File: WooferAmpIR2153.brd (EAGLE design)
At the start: 142.2 x 47.3 mm, 71 parts

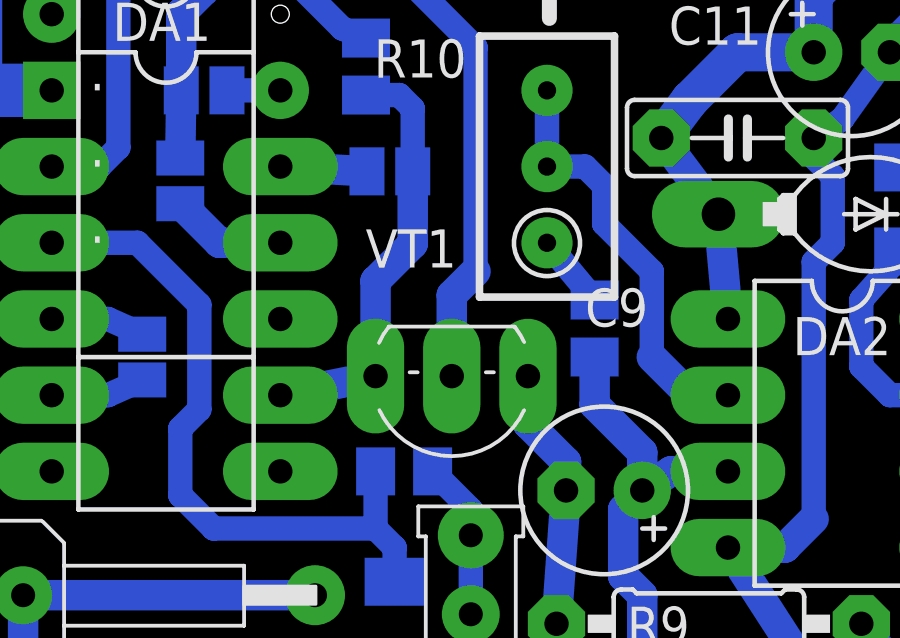
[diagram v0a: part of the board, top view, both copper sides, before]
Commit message: rel4
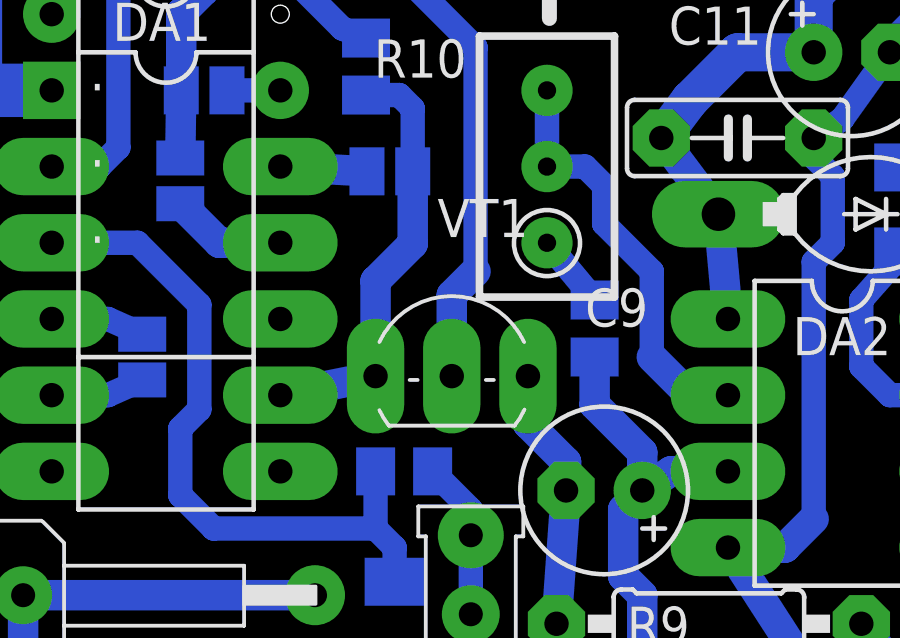
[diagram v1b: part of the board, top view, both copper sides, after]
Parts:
- VT1: device transistor:TO92-CBE -> m_transistor:TO92
- moved VT1 1.27 mm to (26.4, 17.1), turned to 0 degrees
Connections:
- net CO: now also VT1.1; no longer VT1.E
- net GND: now also VT1.2; no longer VT1.B
- net N$50: now also VT1.3; no longer VT1.C
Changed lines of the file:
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@@
 </autorouter>
 <elements>
-<element name="VT1" library="transistor" package="TO92-CBE" value="2N5401" x="26.3525" y="15.875" smashed="yes" rot="R180">
-<attribute name="NAME" x="26.51125" y="20.7645" size="1.27" layer="25" ratio="10" rot="R180"/>
-<attribute name="VALUE" x="23.1775" y="17.9705" size="1.27" layer="27" ratio="10"/>
+<element name="VT1" library="m_transistor" package="TO92" value="2N5401" x="26.3525" y="17.145" smashed="yes">
+<attribute name="NAME" x="25.87625" y="20.5105" size="1.27" layer="25" ratio="10"/>
+<attribute name="VALUE" x="29.5275" y="15.0495" size="1.27" layer="27" ratio="10" rot="R180"/>
 </element>
 <element name="C10" library="resistor" package="C075-032X103" value="750" x="35.2425" y="4.7625" smashed="yes">
@@
 <element name="R11" library="resistor" package="M0805" value="750" x="31.115" y="17.4625" smashed="yes" rot="MR270">
 <attribute name="NAME" x="26.63825" y="18.95475" size="1.27" layer="26" ratio="10" rot="MR180"/>
-<attribute name="VALUE" x="26.0731" y="17.78" size="1.27" layer="28" ratio="10" rot="MR0"/>
+<attribute name="VALUE" x="26.0731" y="18.0975" size="1.27" layer="28" ratio="10" rot="MR0"/>
 </element>
 <element name="C11" library="resistor" package="C050-025X075" value="100n" x="35.8775" y="23.8125" smashed="yes">
@@
 <contactref element="C17" pad="2"/>
 <contactref element="VT2" pad="2"/>
-<contactref element="VT1" pad="B"/>
+<contactref element="VT1" pad="2"/>
 <contactref element="R12" pad="1"/>
 <contactref element="C3" pad="1"/>
@@
 </signal>
 <signal name="N$50">
-<contactref element="VT1" pad="C"/>
+<contactref element="VT1" pad="3"/>
 <contactref element="R9" pad="1"/>
 <contactref element="C9" pad="-"/>
@@
 <contactref element="R8" pad="1"/>
 <contactref element="SJ3" pad="2"/>
-<contactref element="VT1" pad="E"/>
+<contactref element="VT1" pad="1"/>
 <contactref element="DA1" pad="9"/>
 <wire x1="20.6375" y1="15.24" x2="23.8125" y2="15.875" width="1.016" layer="16"/>
